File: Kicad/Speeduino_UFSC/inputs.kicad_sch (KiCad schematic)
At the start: 41 parts, among them IC1 Trig Cond Socket, U3 MPX4250, U4 SP721, U5 SP721

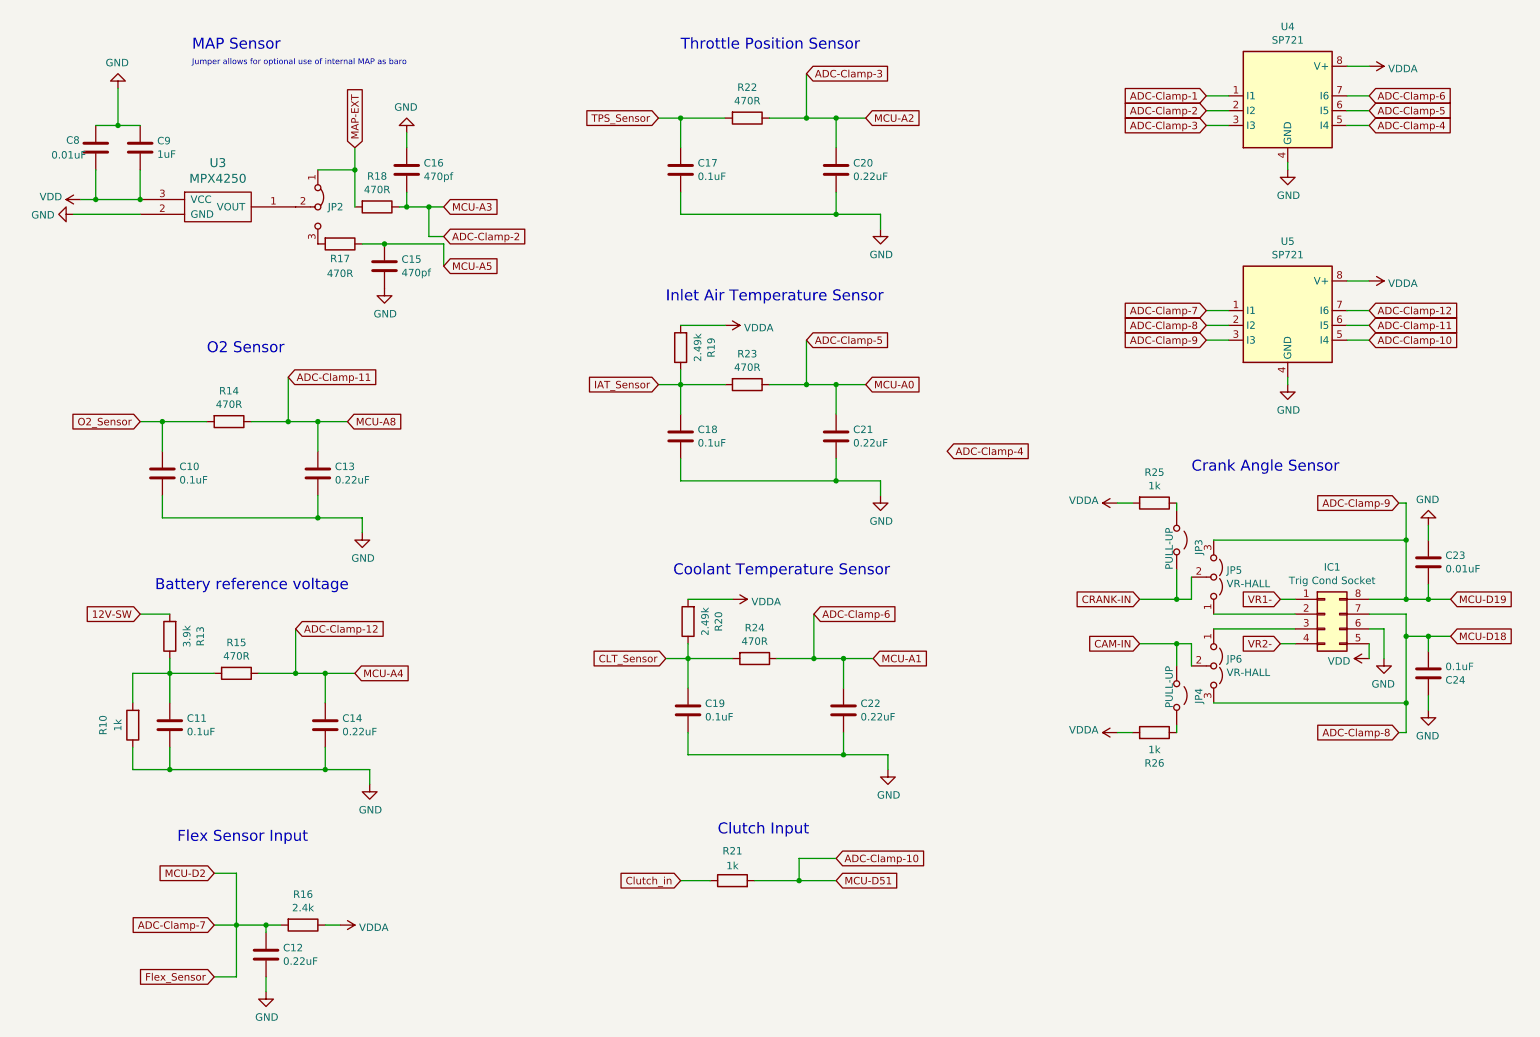
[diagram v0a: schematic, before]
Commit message: Update Kicad
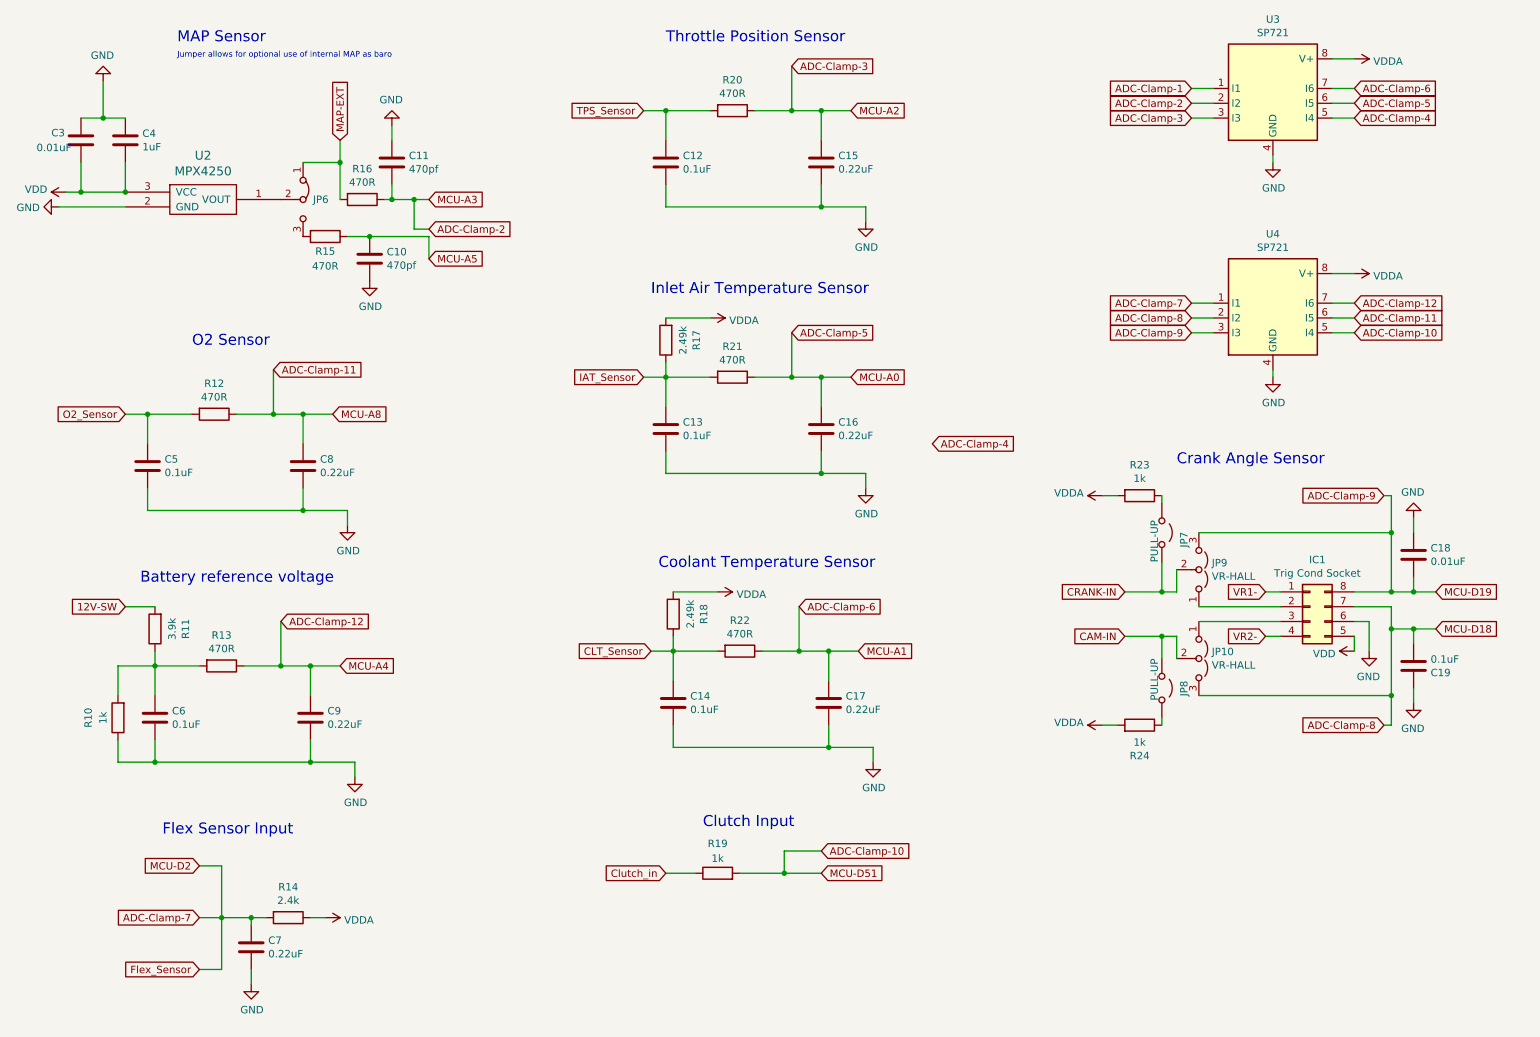
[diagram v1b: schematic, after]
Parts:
- removed C20, C21, C22: 0.22uF, Capacitor_THT:C_Disc_D5.0mm_W2.5mm_P2.50mm, symbol Device:C
- removed C23: 0.01uF, Capacitor_THT:C_Disc_D5.0mm_W2.5mm_P2.50mm, symbol Device:C
- removed C24: 0.1uF, Capacitor_THT:C_Disc_D5.0mm_W2.5mm_P2.50mm, symbol Device:C
- removed JP2: Jumper_3_Bridged12, Jumper:SolderJumper-3_P1.3mm_Bridged12_RoundedPad1.0x1.5mm, symbol Jumper:Jumper_3_Bridged12
- removed JP3, JP4: PULL-UP, Connector_PinHeader_2.54mm:PinHeader_1x02_P2.54mm_Vertical, symbol Jumper:Jumper_2_Open
- removed JP5, JP6: VR-HALL, Connector_PinHeader_2.54mm:PinHeader_1x03_P2.54mm_Vertical, symbol Jumper:Jumper_3_Open
- removed R25, R26: 1k, Resistor_THT:R_Axial_DIN0204_L3.6mm_D1.6mm_P5.08mm_Horizontal, symbol Device:R
- removed U3: MPX4250, Misc:MPX4250, symbol v0.4.3d-rescue:MPX4250-Misc-v0.4.4c-rescue
- removed U5: SP721, Package_DIP:DIP-8_W7.62mm, symbol IC_Automotive:SP721
- added C3: 0.01uF, Capacitor_THT:C_Disc_D5.0mm_W2.5mm_P2.50mm, symbol Device:C
- added C4: 1uF, Capacitor_THT:C_Disc_D5.0mm_W2.5mm_P2.50mm, symbol Device:C
- added C5, C6: 0.1uF, Capacitor_THT:C_Disc_D5.0mm_W2.5mm_P2.50mm, symbol Device:C
- added C7: 0.22uF, Capacitor_THT:C_Disc_D5.0mm_W2.5mm_P2.50mm, symbol Device:C
- added JP10, JP9: VR-HALL, Connector_PinHeader_2.54mm:PinHeader_1x03_P2.54mm_Vertical, symbol Jumper:Jumper_3_Open
- added JP6: Jumper_3_Bridged12, Jumper:SolderJumper-3_P1.3mm_Bridged12_RoundedPad1.0x1.5mm, symbol Jumper:Jumper_3_Bridged12
- added JP7, JP8: PULL-UP, Connector_PinHeader_2.54mm:PinHeader_1x02_P2.54mm_Vertical, symbol Jumper:Jumper_2_Open
- added R11: 3.9k, Resistor_THT:R_Axial_DIN0204_L3.6mm_D1.6mm_P5.08mm_Horizontal, symbol Device:R
- added R12: 470R, Resistor_THT:R_Axial_DIN0204_L3.6mm_D1.6mm_P5.08mm_Horizontal, symbol Device:R
- added U2: MPX4250, Misc:MPX4250, symbol v0.4.3d-rescue:MPX4250-Misc-v0.4.4c-rescue
- added U3: SP721, Package_DIP:DIP-8_W7.62mm, symbol IC_Automotive:SP721
- C10, C11: value 0.1uF -> 470pf; Digikey Part Number 445-180563-1-ND -> 445-180522-1-ND; Manufacturer_Part_Number FA18X8R1E104KNU06 -> FA18NP01H471JNU06; URL https://www.digikey.com.au/product-detail/en/tdk-corporation/FA18X8R1E104KNU06/445-180563-1-ND/9560689 -> https://www.digikey.com.au/product-detail/en/tdk-corporation/FA18NP01H471JNU06/445-180522-1-ND/9560648
- C12, C13, C14: value 0.22uF -> 0.1uF; Digikey Part Number 445-180564-1-ND -> 445-180563-1-ND; Manufacturer_Part_Number FA18X8R1E224KRU06 -> FA18X8R1E104KNU06; URL https://www.digikey.com.au/product-detail/en/tdk-corporation/FA18X8R1E224KRU06/445-180564-1-ND/9560690 -> https://www.digikey.com.au/product-detail/en/tdk-corporation/FA18X8R1E104KNU06/445-180563-1-ND/9560689
- C15, C16: value 470pf -> 0.22uF; Digikey Part Number 445-180522-1-ND -> 445-180564-1-ND; Manufacturer_Part_Number FA18NP01H471JNU06 -> FA18X8R1E224KRU06; URL https://www.digikey.com.au/product-detail/en/tdk-corporation/FA18NP01H471JNU06/445-180522-1-ND/9560648 -> https://www.digikey.com.au/product-detail/en/tdk-corporation/FA18X8R1E224KRU06/445-180564-1-ND/9560690
- C17: value 0.1uF -> 0.22uF; Digikey Part Number 445-180563-1-ND -> 445-180564-1-ND; Manufacturer_Part_Number FA18X8R1E104KNU06 -> FA18X8R1E224KRU06; URL https://www.digikey.com.au/product-detail/en/tdk-corporation/FA18X8R1E104KNU06/445-180563-1-ND/9560689 -> https://www.digikey.com.au/product-detail/en/tdk-corporation/FA18X8R1E224KRU06/445-180564-1-ND/9560690
- C18: value 0.1uF -> 0.01uF; Digikey Part Number 445-180563-1-ND -> 445-174244-1-ND; Manufacturer_Part_Number FA18X8R1E104KNU06 -> FA18X7R1H103KNU06; URL https://www.digikey.com.au/product-detail/en/tdk-corporation/FA18X8R1E104KNU06/445-180563-1-ND/9560689 -> https://www.digikey.com.au/product-detail/en/tdk-corporation/FA18X7R1H103KNU06/445-174244-1-ND/5865002
- C8: value 0.01uF -> 0.22uF; Digikey Part Number 445-174244-1-ND -> 445-180564-1-ND; Manufacturer_Part_Number FA18X7R1H103KNU06 -> FA18X8R1E224KRU06; URL https://www.digikey.com.au/product-detail/en/tdk-corporation/FA18X7R1H103KNU06/445-174244-1-ND/5865002 -> https://www.digikey.com.au/product-detail/en/tdk-corporation/FA18X8R1E224KRU06/445-180564-1-ND/9560690
- C9: value 1uF -> 0.22uF; Digikey Part Number 445-180543-1-ND -> 445-180564-1-ND; Manufacturer_Part_Number FA18X7R1E105KRU06 -> FA18X8R1E224KRU06; URL https://www.digikey.com.au/product-detail/en/tdk-corporation/FA18X7R1E105KRU06/445-180543-1-ND/9560669 -> https://www.digikey.com.au/product-detail/en/tdk-corporation/FA18X8R1E224KRU06/445-180564-1-ND/9560690
- R13: value 3.9k -> 470R; Digikey Part Number BC3272CT-ND -> BC3516CT-ND; Manufacturer_Part_Number MBA02040C3901FCT00 -> MBA02040C4700FRP00; URL https://www.digikey.com.au/product-detail/en/vishay-beyschlag-draloric-bc-components/MBA02040C3901FCT00/BC3272CT-ND/6138775 -> https://www.digikey.com.au/product-detail/en/vishay-beyschlag-draloric-bc-components/MBA02040C4700FRP00/BC3516CT-ND/7350946
- R14: value 470R -> 2.4k; Digikey Part Number BC3516CT-ND -> BC3483CT-ND; Manufacturer_Part_Number MBA02040C4700FRP00 -> MBA02040C2401FC100; URL https://www.digikey.com.au/product-detail/en/vishay-beyschlag-draloric-bc-components/MBA02040C4700FRP00/BC3516CT-ND/7350946 -> https://www.digikey.com.au/product-detail/en/vishay-beyschlag-draloric-bc-components/MBA02040C2401FC100/BC3483CT-ND/7350913
- R16: value 2.4k -> 470R; Digikey Part Number BC3483CT-ND -> BC3516CT-ND; Manufacturer_Part_Number MBA02040C2401FC100 -> MBA02040C4700FRP00; URL https://www.digikey.com.au/product-detail/en/vishay-beyschlag-draloric-bc-components/MBA02040C2401FC100/BC3483CT-ND/7350913 -> https://www.digikey.com.au/product-detail/en/vishay-beyschlag-draloric-bc-components/MBA02040C4700FRP00/BC3516CT-ND/7350946
- R17, R18: value 470R -> 2.49k; Digikey Part Number BC3516CT-ND -> BC2.49KXCT-ND; Manufacturer_Part_Number MBA02040C4700FRP00 -> MBA02040C2491FRP00; URL https://www.digikey.com.au/product-detail/en/vishay-beyschlag-draloric-bc-components/MBA02040C4700FRP00/BC3516CT-ND/7350946 -> https://www.digikey.com.au/product-detail/en/vishay-beyschlag-draloric-bc-components/MBA02040C2491FRP00/BC2-49KXCT-ND/336807
- R19: value 2.49k -> 1k; Digikey Part Number BC2.49KXCT-ND -> BC1.00KXCT-ND; Manufacturer_Part_Number MBA02040C2491FRP00 -> MBA02040C1001FRP00; URL https://www.digikey.com.au/product-detail/en/vishay-beyschl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 -> (none)
- R20: value 2.49k -> 470R; Digikey Part Number BC2.49KXCT-ND -> BC3516CT-ND; Manufacturer_Part_Number MBA02040C2491FRP00 -> MBA02040C4700FRP00; URL https://www.digikey.com.au/product-detail/en/vishay-beyschlag-draloric-bc-components/MBA02040C2491FRP00/BC2-49KXCT-ND/336807 -> https://www.digikey.com.au/product-detail/en/vishay-beyschlag-draloric-bc-components/MBA02040C4700FRP00/BC3516CT-ND/7350946
- R21: value 1k -> 470R; Digikey Part Number BC1.00KXCT-ND -> BC3516CT-ND; Manufacturer_Part_Number MBA02040C1001FRP00 -> MBA02040C4700FRP00; URL (none) -> https://www.digikey.com.au/product-detail/en/vishay-beyschl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
- R23, R24: value 470R -> 1k; Digikey Part Number BC3516CT-ND -> BC1.00KXCT-ND; Manufacturer_Part_Number MBA02040C4700FRP00 -> MBA02040C1001FRP00; URL https://www.digikey.com.au/product-detail/en/vishay-beyschl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 -> (none)
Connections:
- net 12V-SW: now also R11.2; no longer R13.2
- net ADC-Clamp-1: now also U3.1 (I1); no longer U4.1 (I1)
- net ADC-Clamp-10: now also R19.2, U4.5 (I4); no longer R21.2
- net ADC-Clamp-11: now also C8.1, U4.6 (I5), R12.1; no longer C13.1, R14.1
- net ADC-Clamp-12: now also C9.1, R13.1, U4.7 (I6); no longer C14.1, R15.1
- net ADC-Clamp-2: now also C11.2, R16.1, U3.2 (I2); no longer C16.2, R18.1, U4.2 (I2)
- net ADC-Clamp-3: now also C15.1, R20.1, U3.3 (I3); no longer R22.1, U4.3 (I3)
- net ADC-Clamp-4: now also U3.5 (I4); no longer U4.5 (I4)
- net ADC-Clamp-5: now also C16.1, R21.1, U3.6 (I5); no longer R23.1, U4.6 (I5)
- net ADC-Clamp-6: now also C17.1, R22.1, U3.7 (I6); no longer R24.1, U4.7 (I6)
- net ADC-Clamp-7: now also R14.2, U4.1 (I1), C7.1; no longer C12.1, R16.2
- net ADC-Clamp-8: now also C19.2, U4.2 (I2), JP10.3 (B)
- net ADC-Clamp-9: now also C18.2, U4.3 (I3), JP9.3 (B)
- net CAM-IN: now also JP10.2 (C), JP8.1 (A)
- net CLT_Sensor: now also C14.1, R18.1, R22.2; no longer C19.1, R20.1, R24.2
- net CRANK-IN: now also JP7.1 (A), JP9.2 (C)
- net Clutch_in: now also R19.1; no longer R21.1
- net GND: now also C11.1, C16.2, C18.1, C19.1, C8.2, C9.2, C3.1, C4.1, C5.2, C6.2, C7.2, U2.2 (GND), U3.4 (GND); no longer C11.2, C16.1, C18.2, C19.2, C8.1, C9.1
- net IAT_Sensor: now also C13.1, R17.1, R21.2; no longer C18.1, R19.1, R23.2
- net MAP-EXT: now also R16.2, JP6.1 (A); no longer R18.2
- net MCU-A5: now also C10.1, R15.1; no longer C15.1, R17.1
- net O2_Sensor: now also C5.1, R12.2; no longer C10.1, R14.2
- net TPS_Sensor: now also C12.1, R20.2; no longer C17.1, R22.2
- net VDD: now also C3.2, C4.2, U2.3 (VCC); no longer C8.2, C9.2
- net VDDA: now also R14.1, R17.2, R18.2, R23.2, R24.2, U3.8 (V+); no longer R16.1, R19.2, R20.2
- net at IC1.3 (Pin_3): now also JP10.1 (A)
- net at IC1.2 (Pin_2): now also JP9.1 (A)
- new net: JP8.2 (B), R24.1
- new net: C6.1, R10.2, R11.1, R13.2
- new net: JP7.2 (B), R23.1
- new net: JP6.2 (C), U2.1 (VOUT)
- new net: JP6.3 (B), R15.2
